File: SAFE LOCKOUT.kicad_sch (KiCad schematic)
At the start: 42 parts, among them J1 Conn_01x08_Pin, J10 Conn_01x02_Pin, J2 Conn_01x02_Pin, J3 Conn_01x02_Pin, J4 Conn_01x02_Pin, J5 Conn_01x02_Pin, J6 Conn_01x02_Pin, J7 Conn_01x02_Pin, J8 Conn_01x02_Pin, J9 Conn_01x02_Pin, K1 PR30-24V-450-1A, Q1 BSS138, Q2 BSS138, Q3 BSS138, Q4 BSS138, Q5 BSS138, Q6 BSS138, Q7 BSS138, Q8 BSS138

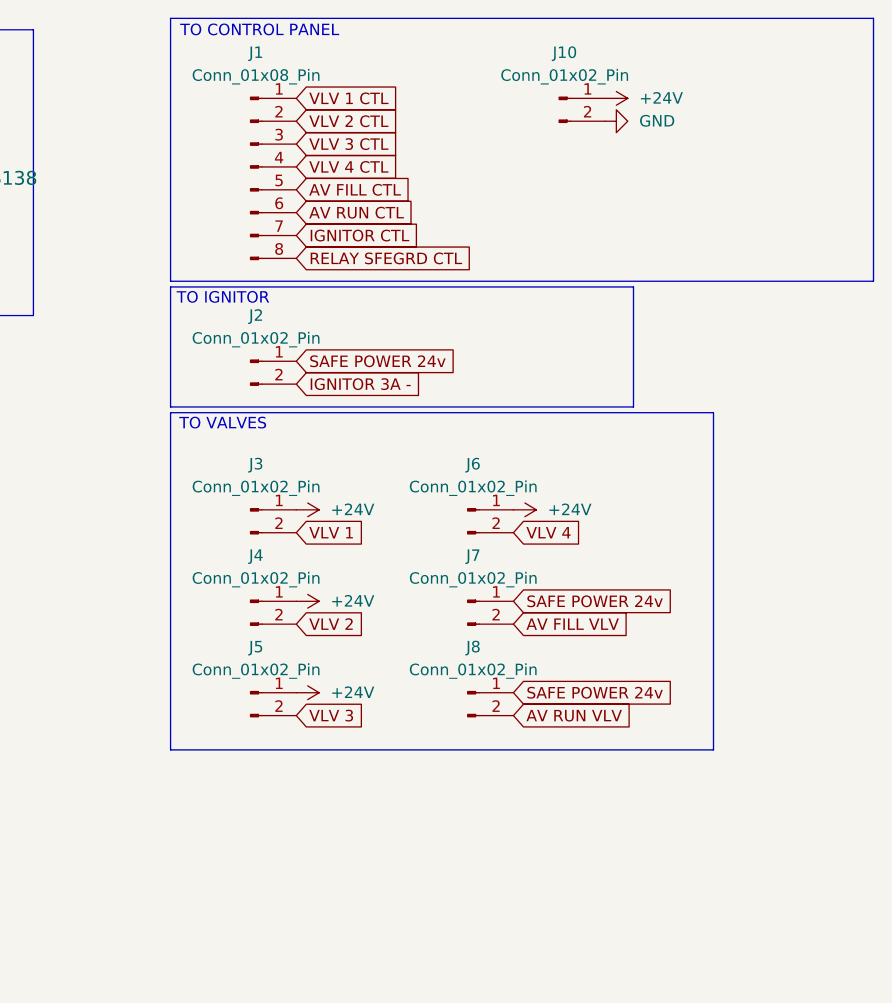
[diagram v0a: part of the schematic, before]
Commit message: logan did pcb, some suff still needs to be fixed
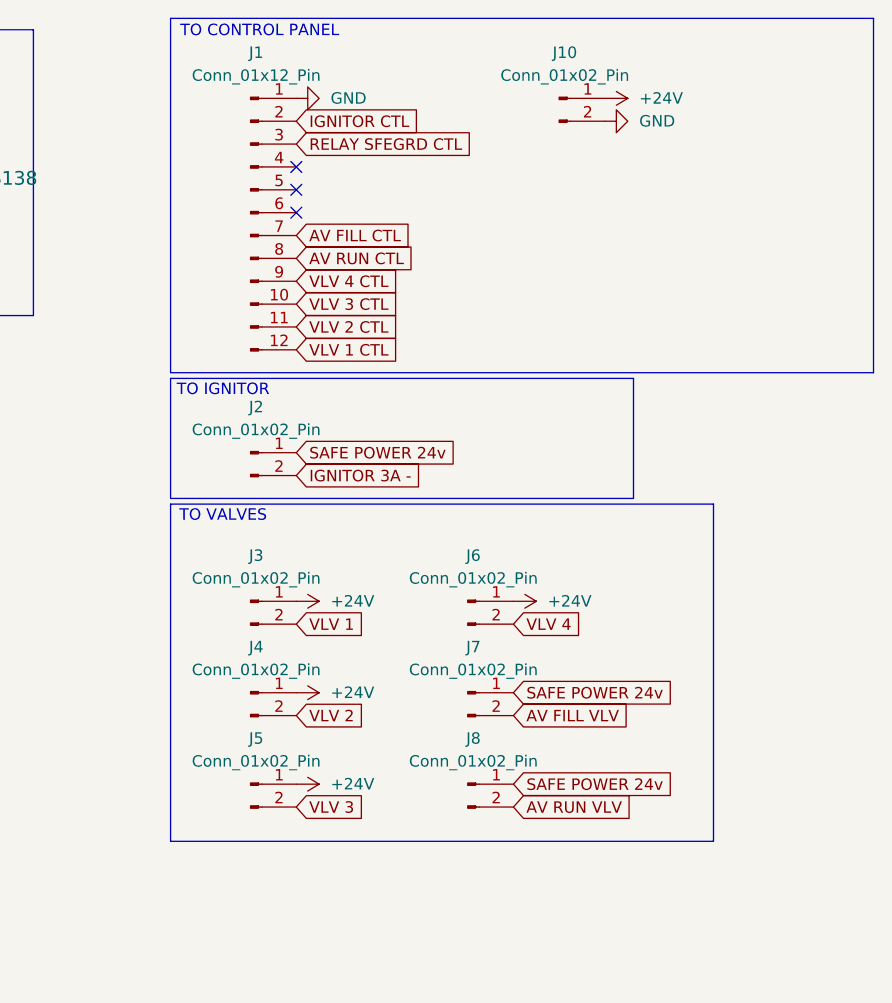
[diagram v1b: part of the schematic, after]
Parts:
- removed J1: Conn_01x08_Pin, Connector_Molex:Molex_Micro-Fit_3.0_43045-1600_2x08_P3.00mm_Horizontal, symbol Connector:Conn_01x08_Pin
- added J1: Conn_01x12_Pin, 430451200:MOLEX_430451200, symbol Connector:Conn_01x12_Pin
- D1, D2, D3, D4, D5, D6, D7: footprint digikey-footprints:DO-214AC -> Solenoid Safeguard:DO-214AC
- J2: footprint Connector_JST:JST_XH_B2B-XH-AM_1x02_P2.50mm_Vertical -> Connector_Molex:Molex_Micro-Fit_3.0_43650-0200_1x02_P3.00mm_Horizontal
- J9: footprint Connector_Phoenix_MSTB:PhoenixContact_MSTBVA_2,5_2-G_1x02_P5.00mm_Vertical -> Kinky:PhoenixContact_MSTBVA_2,5_2-G_1x02_P5.00mm_Vertical
- K1: footprint PR30_24V_450_1A:RELAY_PR30-24V-450-1A -> Solenoid Safeguard:RELAY_PR30-24V-450-1A
- Q1, Q2, Q3, Q4, Q5, Q6, Q7, Q8: footprint digikey-footprints:SOT-23-3 -> Package_TO_SOT_SMD:SOT-23-3
- R1, R11, R13, R15, R3, R5, R7, R9: footprint PCM_JLCPCB:R_0805 -> Solenoid Safeguard:R_0805
- R10, R12, R14, R16, R2, R4, R6, R8: footprint Resistor_SMD:R_0402_1005Metric -> Solenoid Safeguard:R_0805
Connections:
- net AV  RUN CTL: now also J1.8 (Pin_8)
- net AV FILL CTL: now also J1.7 (Pin_7)
- net GND: now also J1.1 (Pin_1)
- net IGNITOR CTL: now also J1.2 (Pin_2)
- net RELAY SFEGRD CTL: now also J1.3 (Pin_3)
- net VLV 1 CTL: now also J1.12 (Pin_12)
- net VLV 2 CTL: now also J1.11 (Pin_11)
- net VLV 3 CTL: now also J1.10 (Pin_10)
- net VLV 4 CTL: now also J1.9 (Pin_9)
- no-connect marks 0 -> 3
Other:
- moved on the sheet: J2, J3, J4, J5, J6, J7, J8
